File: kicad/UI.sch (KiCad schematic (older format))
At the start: 13 parts, among them Q4 BSS138, SW3 BUTTON

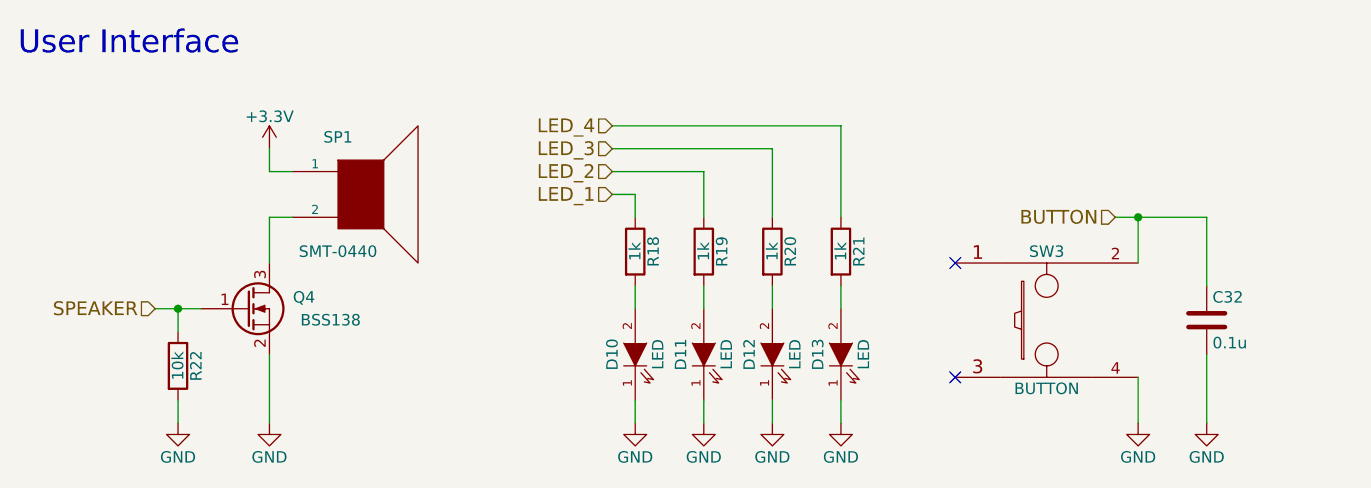
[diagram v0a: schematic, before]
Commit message: 新基板，部品を配置
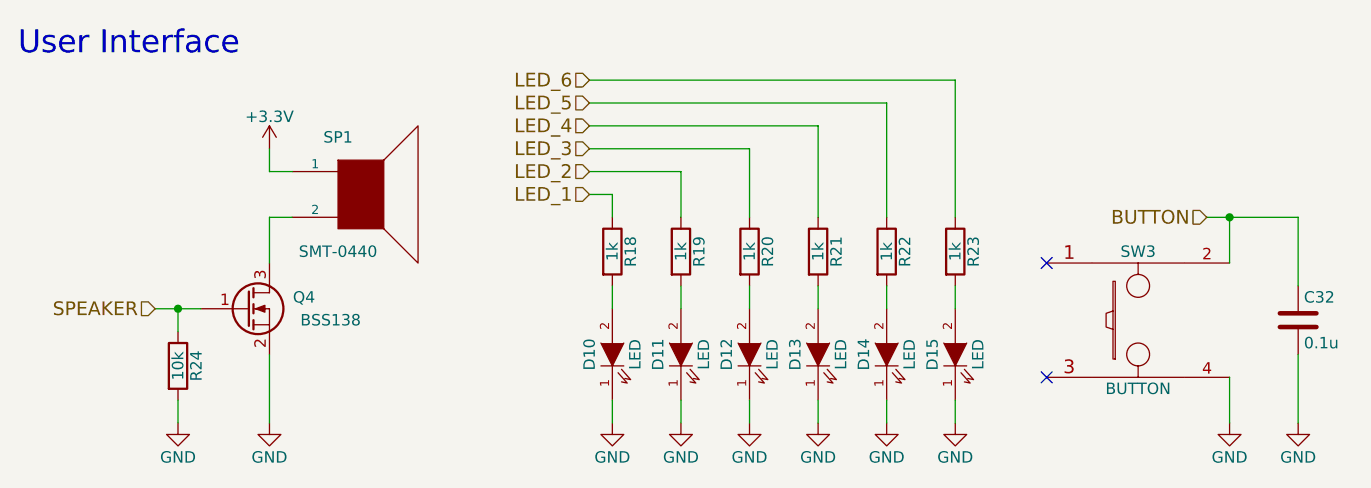
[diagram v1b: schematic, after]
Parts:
- added D14, D15: LED, LEDs:LED_0603, symbol LED
- added R22, R23: 1k, Resistors_SMD:R_0402, symbol R
- renumbered R22 to R24
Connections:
- net GND: now also D14.1 (K), D15.1 (K)
- new net: D14.2 (A), R22.2
- new net: D15.2 (A), R23.2
- new net LED_5: R22.1
- new net LED_6: R23.1
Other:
- moved on the sheet: C32, D10, D11, D12, D13, R18, R19, R20, R21, SW3
